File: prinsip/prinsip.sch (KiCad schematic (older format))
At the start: 21 parts, among them SW1 SW_MEC_5G, SW2 SW_DPDT_x2, SW2 SW_MEC_5G, SW3 SW_MEC_5G, SW4 SW_MEC_5G, SW5 SW_MEC_5G, U1 ATmega8515L-8JU, U2 TM1637, U3 CA56-12CGKWA, U4 MCP23S17_SO, U5 MAX232, U6 ATmega8515L-8JU, U7 74LS373, U8 6264

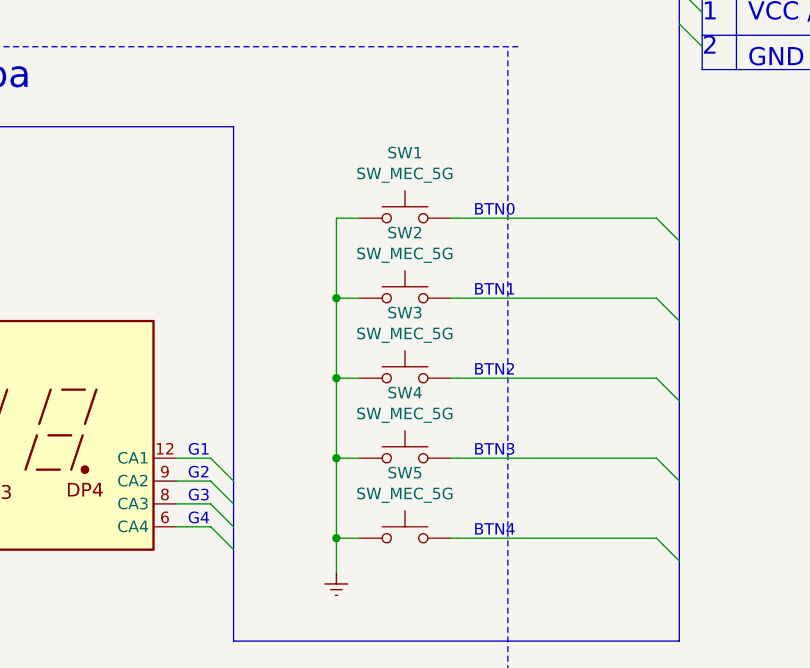
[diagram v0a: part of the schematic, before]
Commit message: update prinsip
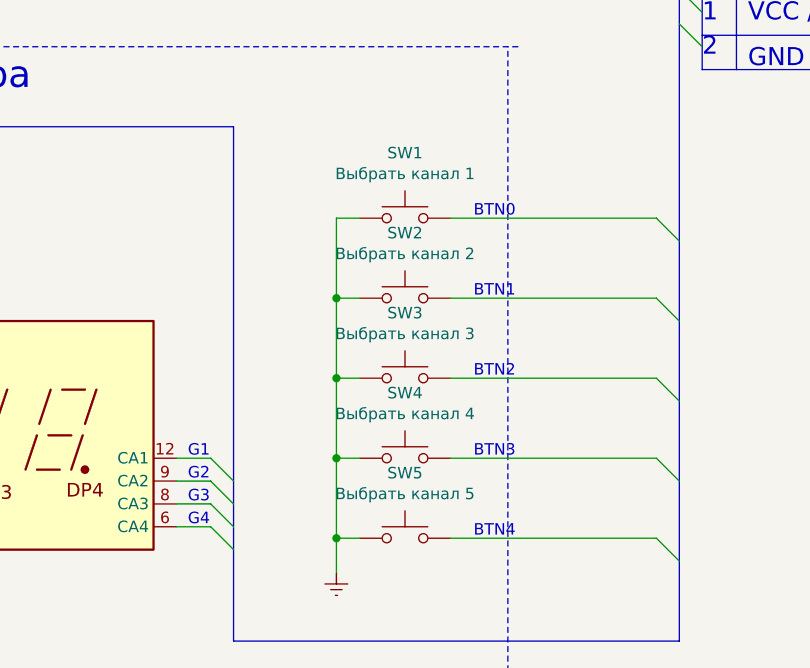
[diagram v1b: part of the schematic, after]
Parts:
- SW1: value SW_MEC_5G -> Выбрать канал 1
- SW2: value SW_MEC_5G -> Выбрать канал 2
- SW3: value SW_MEC_5G -> Выбрать канал 3
- SW4: value SW_MEC_5G -> Выбрать канал 4
- SW5: value SW_MEC_5G -> Выбрать канал 5
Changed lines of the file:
@@
 P 7600 8950
 F 0 "SW1" H 7600 9235 50  0000 C CNN
-F 1 "SW_MEC_5G" H 7600 9144 50  0000 C CNN
+F 1 "Выбрать канал 1" H 7600 9144 50  0000 C CNN
 F 2 "" H 7600 9150 50  0001 C CNN
 F 3 "http://www.apem.com/int/index.php?controller=attachment&id_attachment=488" H 7600 9150 50  0001 C CNN
@@
 P 7600 9300
 F 0 "SW2" H 7600 9585 50  0000 C CNN
-F 1 "SW_MEC_5G" H 7600 9494 50  0000 C CNN
+F 1 "Выбрать канал 2" H 7600 9494 50  0000 C CNN
 F 2 "" H 7600 9500 50  0001 C CNN
 F 3 "http://www.apem.com/int/index.php?controller=attachment&id_attachment=488" H 7600 9500 50  0001 C CNN
@@
 P 7600 9650
 F 0 "SW3" H 7600 9935 50  0000 C CNN
-F 1 "SW_MEC_5G" H 7600 9844 50  0000 C CNN
+F 1 "Выбрать канал 3" H 7600 9844 50  0000 C CNN
 F 2 "" H 7600 9850 50  0001 C CNN
 F 3 "http://www.apem.com/int/index.php?controller=attachment&id_attachment=488" H 7600 9850 50  0001 C CNN
@@
 P 7600 10000
 F 0 "SW4" H 7600 10285 50  0000 C CNN
-F 1 "SW_MEC_5G" H 7600 10194 50  0000 C CNN
+F 1 "Выбрать канал 4" H 7600 10194 50  0000 C CNN
 F 2 "" H 7600 10200 50  0001 C CNN
 F 3 "http://www.apem.com/int/index.php?controller=attachment&id_attachment=488" H 7600 10200 50  0001 C CNN
@@
 P 7600 10350
 F 0 "SW5" H 7600 10635 50  0000 C CNN
-F 1 "SW_MEC_5G" H 7600 10544 50  0000 C CNN
+F 1 "Выбрать канал 5" H 7600 10544 50  0000 C CNN
 F 2 "" H 7600 10550 50  0001 C CNN
 F 3 "http://www.apem.com/int/index.php?controller=attachment&id_attachment=488" H 7600 10550 50  0001 C CNN
@@
 Text Notes 14450 3500 0    50   ~ 0
 GND
-Wire Bus Line
-	8900 7800 8900 8300
 $Comp
 L prinsip-rescue:USBASP U?
@@
 Wire Wire Line
 	14850 2450 14850 2600
-Wire Bus Line
-	9150 5350 9150 5650
-Wire Bus Line
-	6350 6750 10050 6750
-Wire Bus Line
-	12600 4450 14350 4450
-Wire Bus Line
-	15950 1800 15950 3000
-Wire Bus Line
-	6850 8550 6850 10800
-Wire Bus Line
-	2550 1800 2550 10850
-Wire Bus Line
-	8800 7400 8800 10800
-Wire Bus Line
-	12600 1600 12600 5950
-Wire Bus Line
-	4200 8550 4200 10850
-Wire Bus Line
-	14350 1800 14350 4450
-Wire Bus Line
-	6350 1800 6350 6750
-Wire Bus Line
-	10050 1600 10050 6750
 Text Notes 14450 2600 0    50   ~ 0
 RST
+Wire Bus Line
+	9150 5350 9150 5650
+Wire Bus Line
+	6350 6750 10050 6750
+Wire Bus Line
+	12600 4450 14350 4450
+Wire Bus Line
+	8900 7800 8900 8300
+Wire Bus Line
+	15950 1800 15950 3000
+Wire Bus Line
+	6850 8550 6850 10800
+Wire Bus Line
+	2550 1800 2550 10850
+Wire Bus Line
+	8800 7400 8800 10800
+Wire Bus Line
+	12600 1600 12600 5950
+Wire Bus Line
+	4200 8550 4200 10850
+Wire Bus Line
+	14350 1800 14350 4450
+Wire Bus Line
+	6350 1800 6350 6750
+Wire Bus Line
+	10050 1600 10050 6750
 $EndSCHEMATC
